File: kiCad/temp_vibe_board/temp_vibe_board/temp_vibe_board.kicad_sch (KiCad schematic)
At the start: 13 parts, among them J1 Conn_01x04_Pin, J9 Conn_01x04_Pin, U1 DEV-13907, U2 MPU-9250, U3 MPU-9250

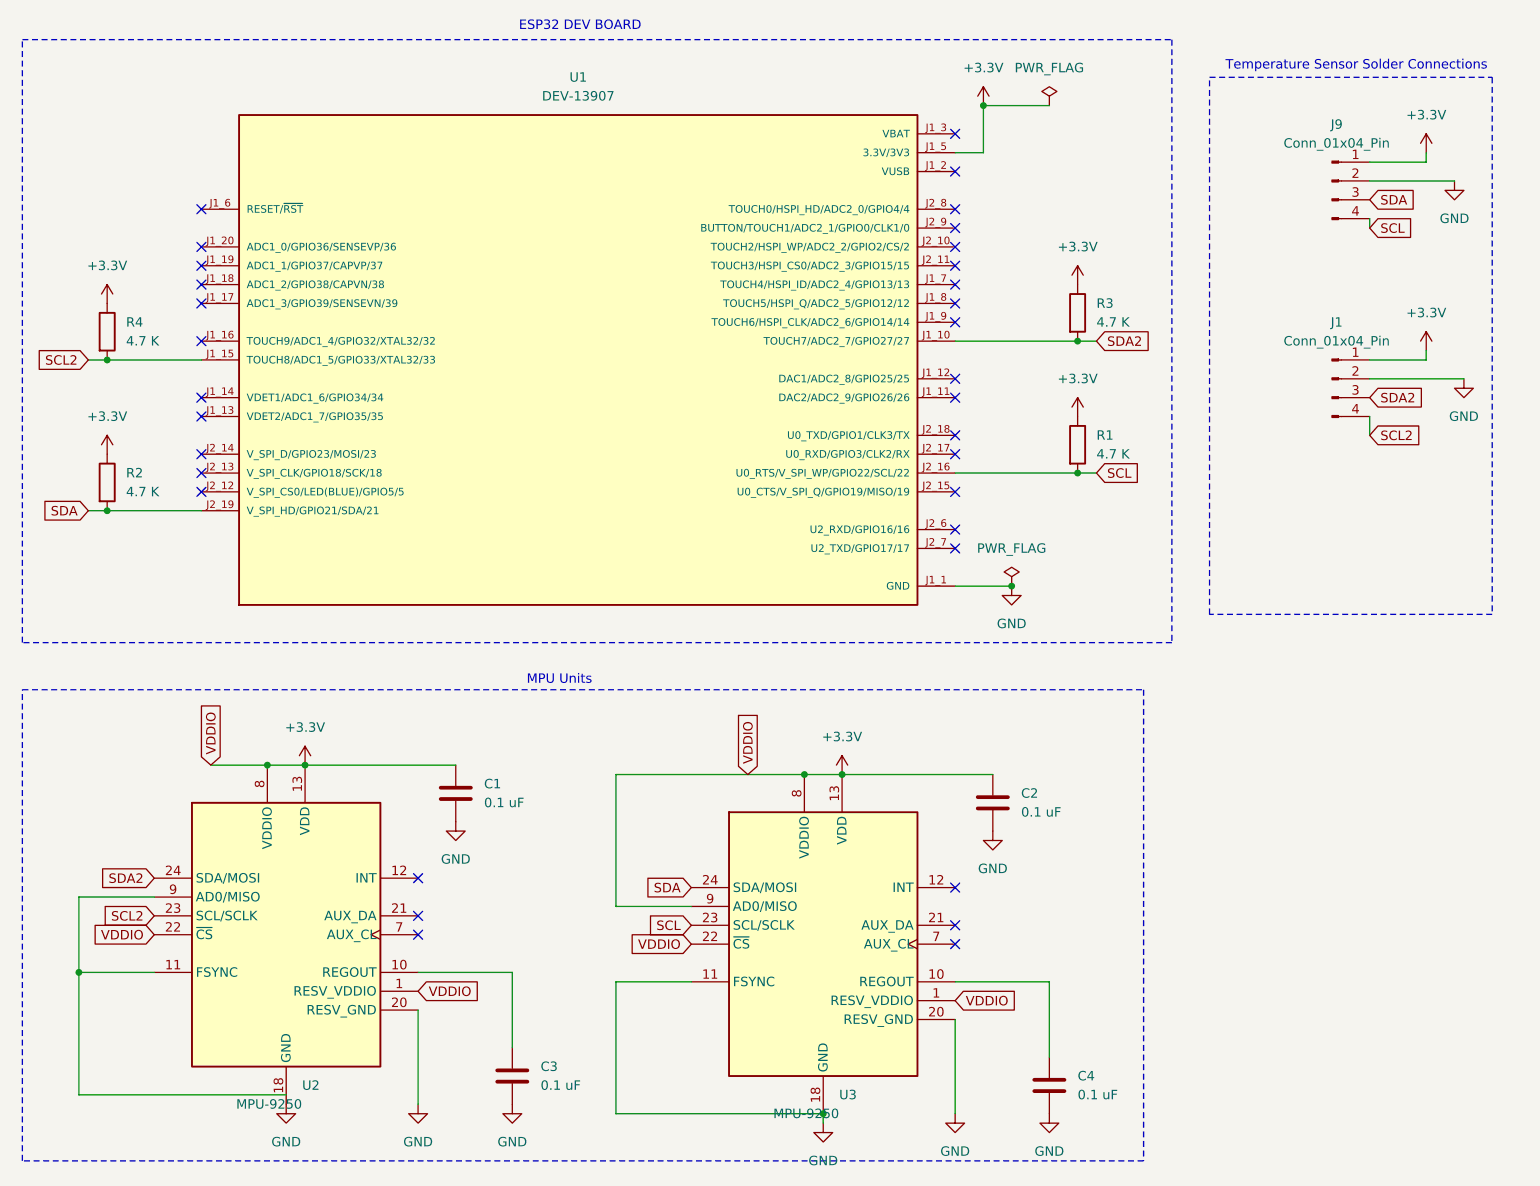
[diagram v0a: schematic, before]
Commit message: MPU6050 PCB
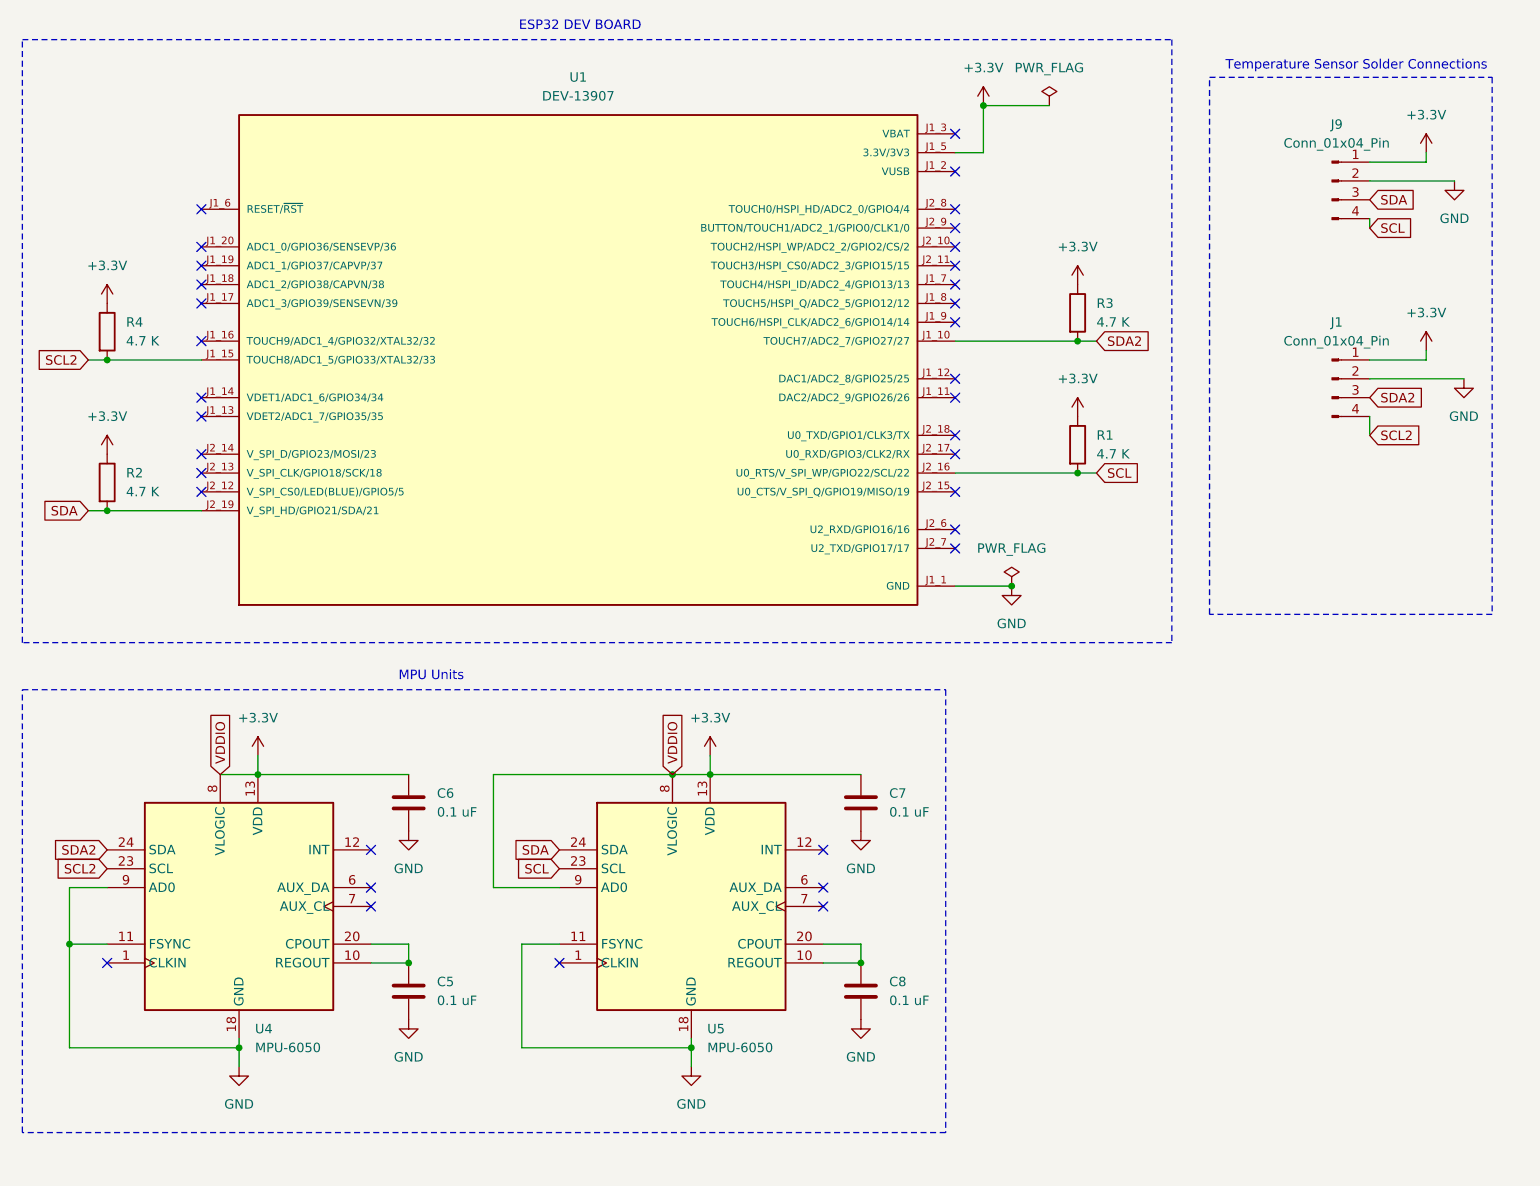
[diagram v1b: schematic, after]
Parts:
- removed C1, C2, C3, C4: 0.1 uF, Capacitor_SMD:C_0805_2012Metric, symbol Device:C
- removed U2, U3: MPU-9250, Sensor_Motion:InvenSense_QFN-24_3x3mm_P0.4mm, symbol Sensor_Motion:MPU-9250
- added C5, C6, C7, C8: 0.1 uF, Capacitor_SMD:C_0805_2012Metric, symbol Device:C
- added U4, U5: MPU-6050, Sensor_Motion:InvenSense_QFN-24_4x4mm_P0.5mm, symbol Sensor_Motion:MPU-6050
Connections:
- net +3.3V: now also C6.1, C7.1, U4.13 (VDD), U4.8 (VLOGIC), U5.13 (VDD), U5.8 (VLOGIC), U5.9 (AD0)
- net GND: now also C5.2, C6.2, C7.2, C8.2, U4.11 (FSYNC), U4.18 (GND), U4.9 (AD0), U5.11 (FSYNC), U5.18 (GND)
- net SCL: now also U5.23 (SCL)
- net SCL2: now also U4.23 (SCL)
- net SDA: now also U5.24 (SDA)
- net SDA2: now also U4.24 (SDA)
- new net: C8.1, U5.10 (REGOUT), U5.20 (CPOUT)
- new net: C5.1, U4.10 (REGOUT), U4.20 (CPOUT)
- no-connect marks 33 -> 35

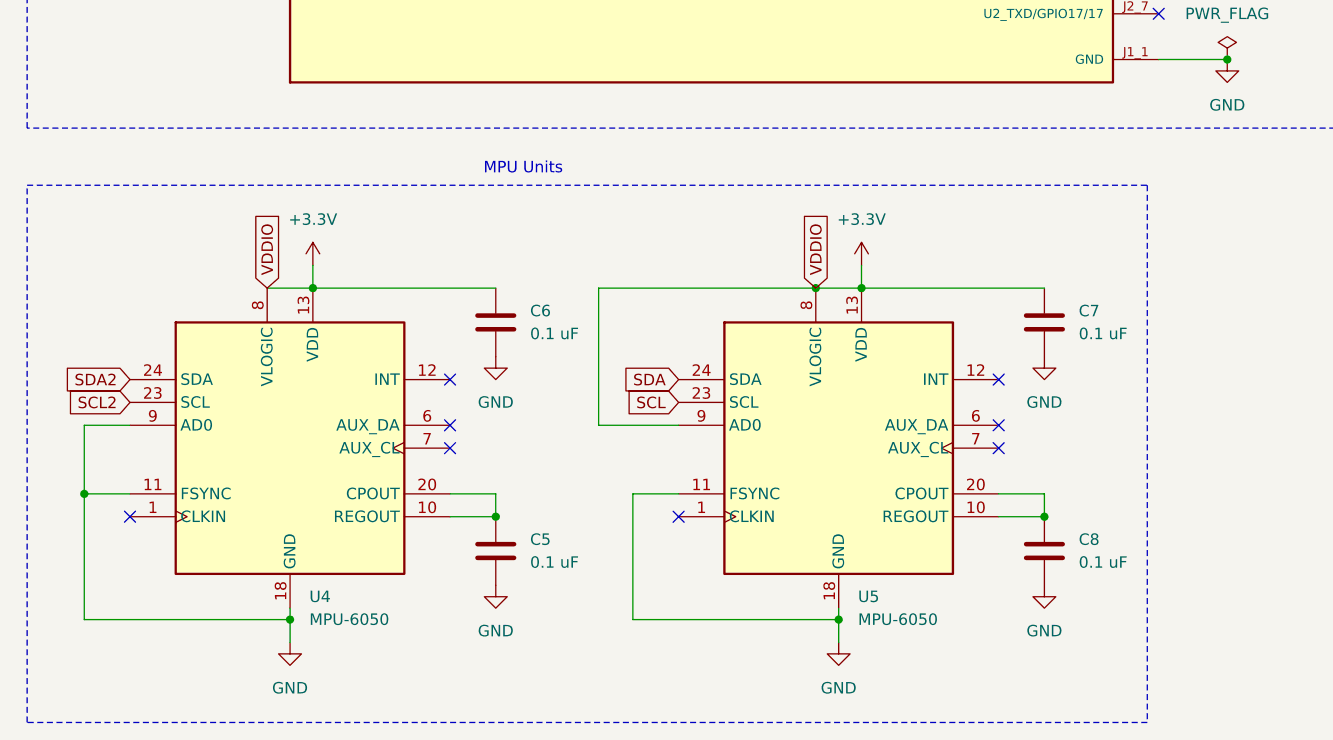
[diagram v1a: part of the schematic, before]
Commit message: fixed sch
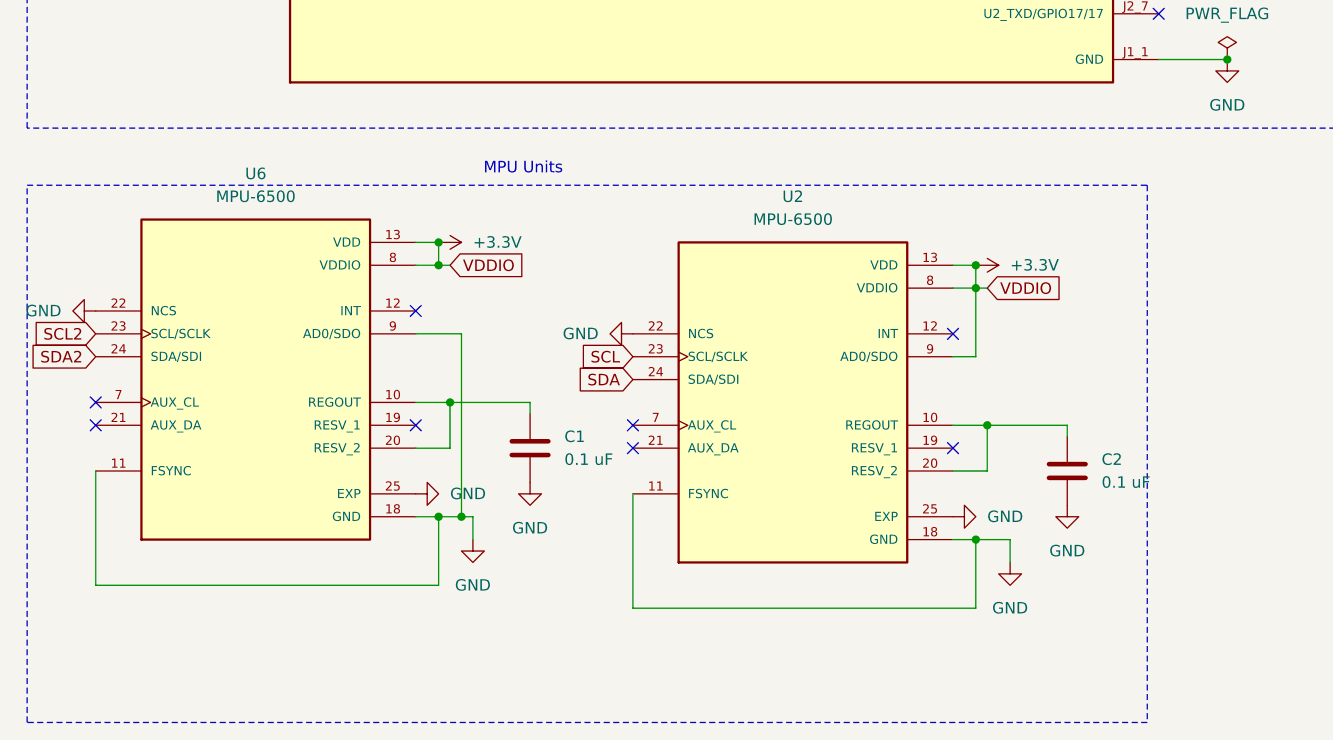
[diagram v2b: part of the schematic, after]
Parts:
- removed C5, C6, C7, C8: 0.1 uF, Capacitor_SMD:C_0805_2012Metric, symbol Device:C
- removed U4, U5: MPU-6050, Sensor_Motion:InvenSense_QFN-24_4x4mm_P0.5mm, symbol Sensor_Motion:MPU-6050
- added C1, C2: 0.1 uF, Capacitor_SMD:C_0805_2012Metric, symbol Device:C
- added U2, U6: MPU-6500, MPU-6500:QFN40P300X300X95-25N, symbol MPU-6500:MPU-6500
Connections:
- net +3.3V: now also U2.13 (VDD), U2.8 (VDDIO), U2.9 (AD0/SDO), U6.13 (VDD), U6.8 (VDDIO)
- net GND: now also C1.2, C2.2, U2.11 (FSYNC), U2.18 (GND), U2.22 (NCS), U2.25 (EXP), U6.11 (FSYNC), U6.18 (GND), U6.22 (NCS), U6.25 (EXP), U6.9 (AD0/SDO)
- net SCL: now also U2.23 (SCL/SCLK)
- net SCL2: now also U6.23 (SCL/SCLK)
- net SDA: now also U2.24 (SDA/SDI)
- net SDA2: now also U6.24 (SDA/SDI)
- new net: C2.1, U2.10 (REGOUT), U2.20 (RESV_2)
- new net: C1.1, U6.10 (REGOUT), U6.20 (RESV_2)
